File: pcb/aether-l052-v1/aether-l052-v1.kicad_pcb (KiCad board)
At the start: 2 copper layers, 50.8 x 22.9 mm, 39 parts, among them J1 USB_C_Receptacle_USB2.0_16P, J2 Conn_01x16_Pin, J3 Conn_01x12_Pin, J4 S2B-PH-SM4-TB, J5 BM04B-SRSS-TB, J6 Conn_ARM_JTAG_SWD_10, Q1 DMG2305UX-7, U1 MCP1711T-3.3I/OT, U2 MCP73832-2-OT, U3 STM32L052K8Ux

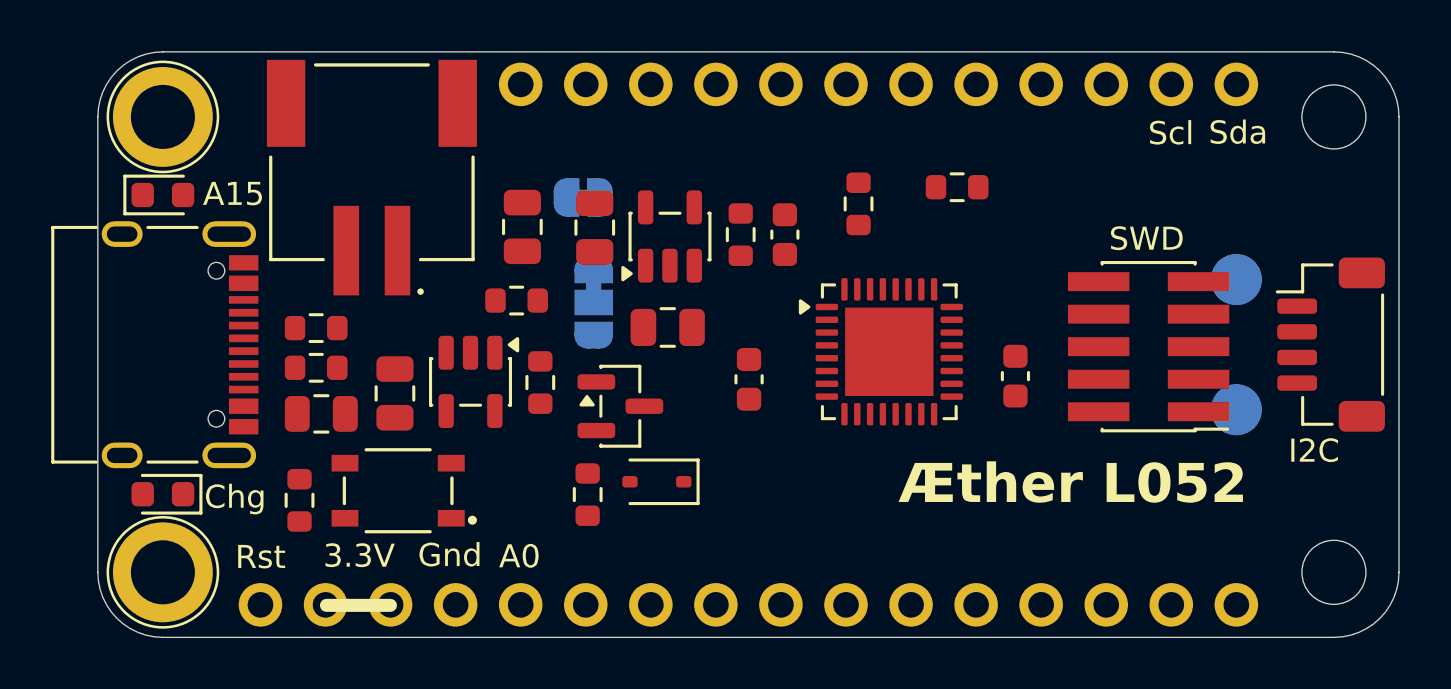
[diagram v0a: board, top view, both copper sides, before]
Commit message: routing
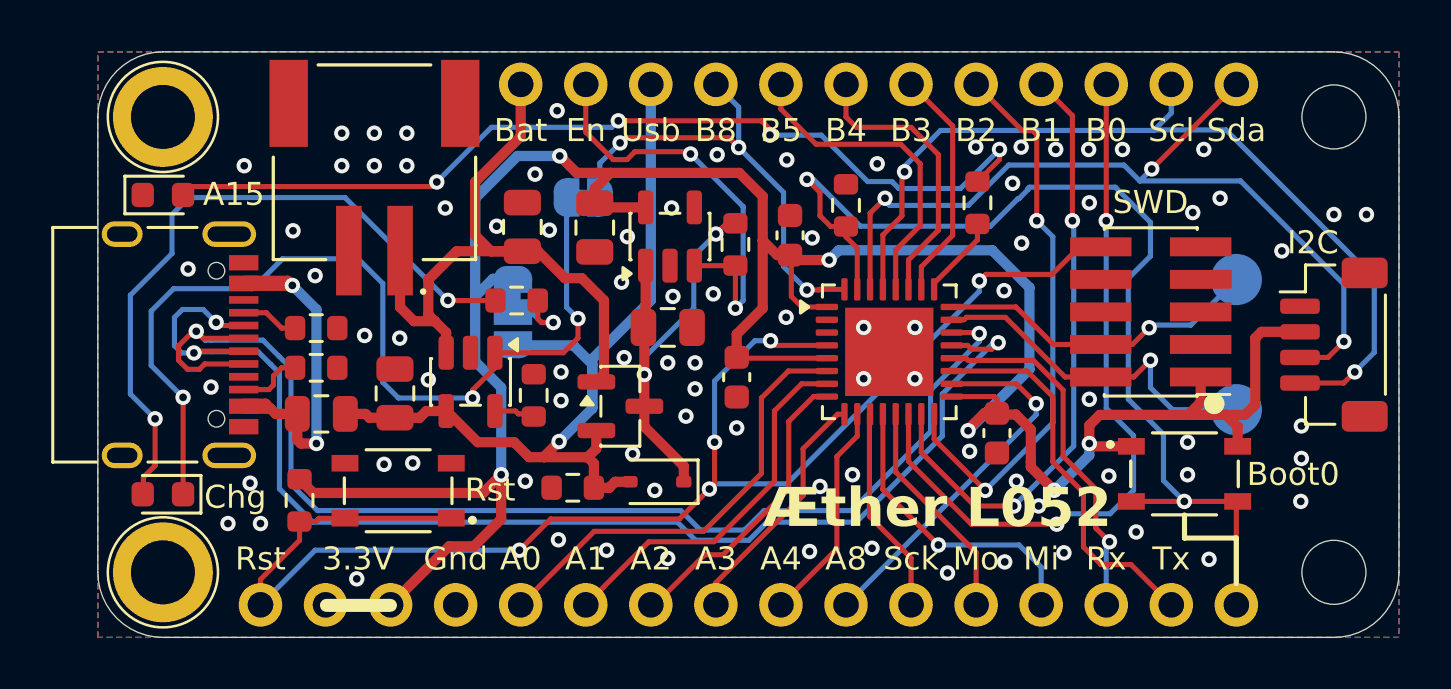
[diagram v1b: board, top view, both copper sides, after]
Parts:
- added S2: SKRPACE010, aether-l052:SKRPACE010, F.Cu at (144.0, 95.2)
- moved TP1 5.08 mm to (146.1, 87.6)
- moved TP2 5.08 mm to (146.1, 92.7)
- moved JP2 3.17 mm to (117.8, 88.9)
- moved C5 2.34 mm to (136.7, 93.6), turned to -90 degrees
- moved J6 1.36 mm to (142.7, 88.9)
- moved R6 1.00 mm to (135.9, 84.6), turned to 90 degrees
- moved R3 0.64 mm to (120.1, 95.8), turned to 180 degrees
- moved R4 0.56 mm to (118.6, 92.2)
- moved R8 0.49 mm to (130.8, 84.7)
- moved C6 0.49 mm to (126.5, 91.4)
- moved R9 0.44 mm to (126.5, 86.3)
- moved C4 0.20 mm to (128.6, 85.9)
- moved J5 0.11 mm to (149.9, 90.2)
- moved J4 0.10 mm to (112.4, 86.5)
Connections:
- J2 pad 2: /A10_USART1_TX -> /A9_USART1_TX
- J2 pad 3: /A9_USART1_RX -> /A10_USART1_RX
- J5 pad 3: /SDA -> /B7_I2C1_SDA
- J5 pad 4: /SCL -> /B6_I2C1_SCL
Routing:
- net VDD: track 0.00 -> 106.6 mm, vias 0 -> 6
- net /!RESET: track 0.00 -> 57.8 mm, vias 0 -> 5
- net /D-: track 0.00 -> 50.3 mm, vias 0 -> 3
- net /D+: track 0.00 -> 48.1 mm, vias 0 -> 2
- net /BOOT0: track 0.00 -> 41.2 mm, vias 0 -> 2
- net Net-(D2-K): track 0.00 -> 36.9 mm, vias 0 -> 3
- net Net-(D3-A): track 0.00 -> 36.6 mm, vias 0 -> 4
- net VBUS: track 0.00 -> 35.9 mm, vias 0 -> 1
- net /B6_I2C1_SCL: track 0.00 -> 34.9 mm, vias 0 -> 2
- net /B7_I2C1_SDA: track 0.00 -> 34.0 mm, vias 0 -> 3
- net /B0: track 0.00 -> 28.5 mm, vias 0 -> 2
- net /VBAT: track 0.00 -> 27.1 mm
- net Net-(D2-A): track 0.00 -> 26.8 mm, vias 0 -> 2
- net /B1: track 0.00 -> 23.9 mm, vias 0 -> 2
- net /B2: track 0.00 -> 22.2 mm, vias 0 -> 2
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- added copper zone on B.Cu, net GND
- added copper zone on F.Cu, net GND
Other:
- board text added: "A1"
- board text added: "A2"
- board text added: "A3"
- board text added: "A4"
- board text added: "A8"
- board text added: "B0"
- board text added: "B1"
- board text added: "B2"
- board text added: "B3"
- board text added: "B4"
- board text added: "B5"
- board text added: "B8"
- board text added: "Bat"
- board text added: "Boot0"
- board text added: "Bt0"
- board text added: "Chg>B8"
- board text added: "ChgPu"
- board text added: "En"
- board text added: "Mi"
- board text added: "Mo"
- board text added: "Rx"
- board text added: "Sck"
- board text added: "Tx"
- board text added: "Usb"
